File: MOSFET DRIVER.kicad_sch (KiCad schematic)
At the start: 46 parts, among them IC1 DRV8302

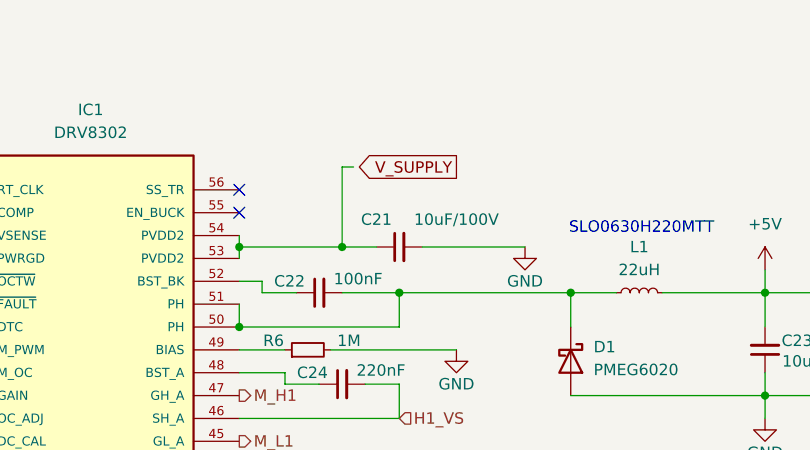
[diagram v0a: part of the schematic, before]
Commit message: ready for review
1. finish routing
2. finish silkscreen adjustment
3. finish DRC and ERC
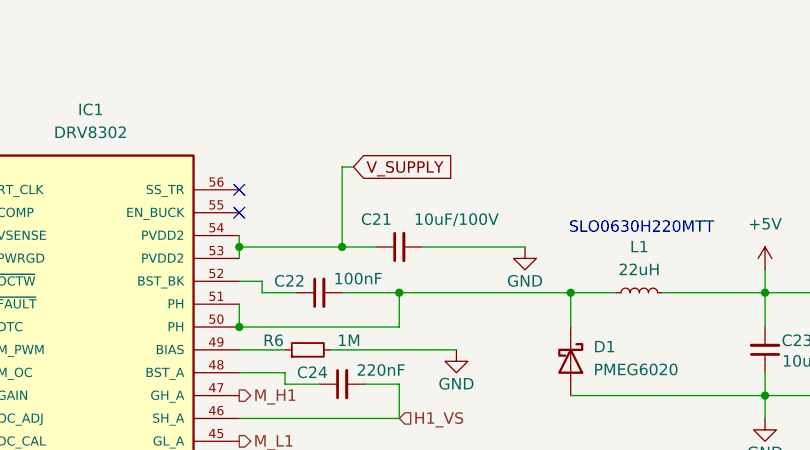
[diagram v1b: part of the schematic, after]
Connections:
- net V_SUPPLY: now also C21.1, IC1.53 (PVDD2), IC1.54 (PVDD2)
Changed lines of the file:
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@@
 	)
 	(global_label "V_SUPPLY"
-		(shape output)
-		(at 143.51 25.4 180)
+		(shape input)
+		(at 132.08 25.4 0)
 		(fields_autoplaced yes)
 		(effects
@@
 				(size 1.27 1.27)
 			)
-			(justify right)
+			(justify left)
 		)
 		(property "Intersheetrefs" "${INTERSHEET_REFS}"
-			(at 131.2719 25.4 0)
+			(at 144.3181 25.4 0)
 			(effects
 				(font
 					(size 1.27 1.27)
 				)
-				(justify right)
+				(justify left)
 				(hide yes)
 			)

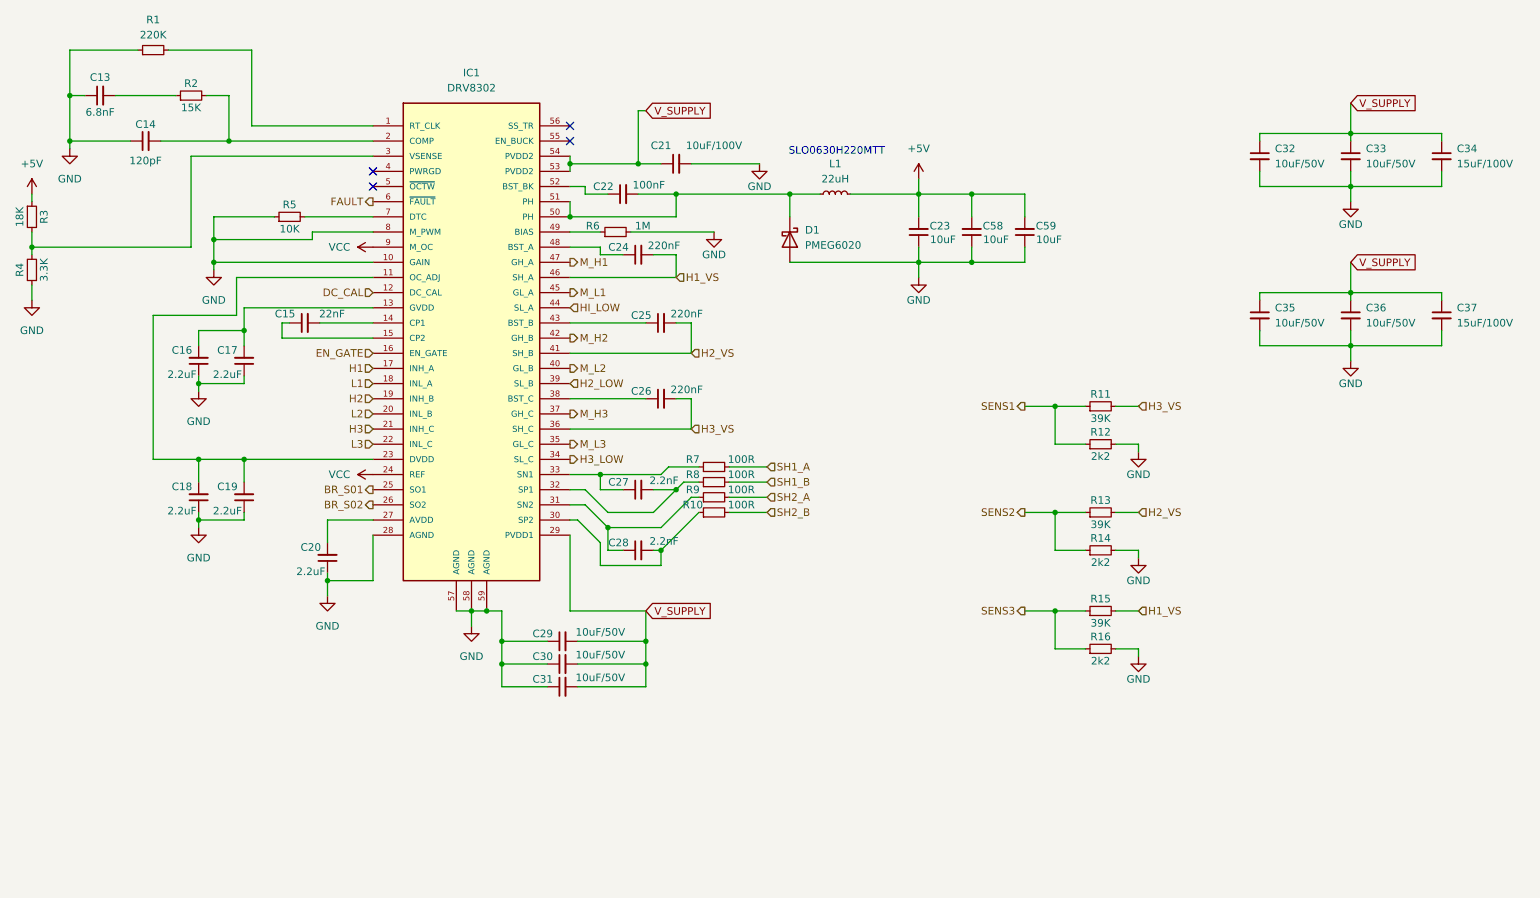
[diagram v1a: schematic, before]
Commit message: finishing+microchecking
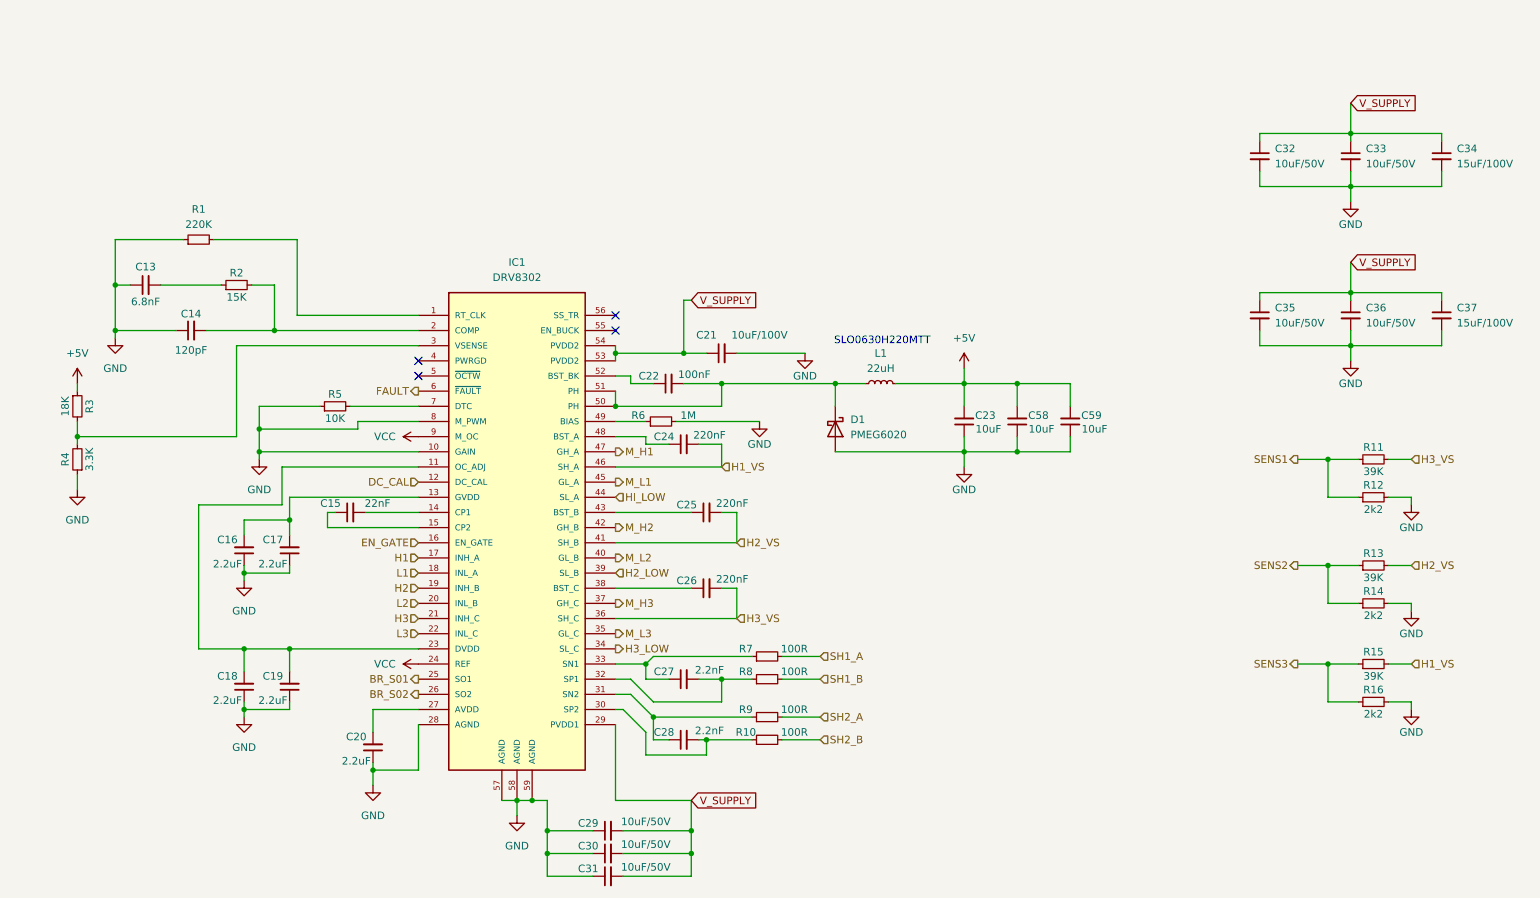
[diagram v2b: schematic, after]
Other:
- moved on the sheet: C13, C14, C15, C16, C17, C18, C19, C20, C21, C22, C23, C24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
